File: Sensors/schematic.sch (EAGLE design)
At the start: 13 parts, among them IC1 LIS331DLHTR, IC2 BMI088, IC3 MCP9803T-M_MS, IC4 MS560702BA03-50

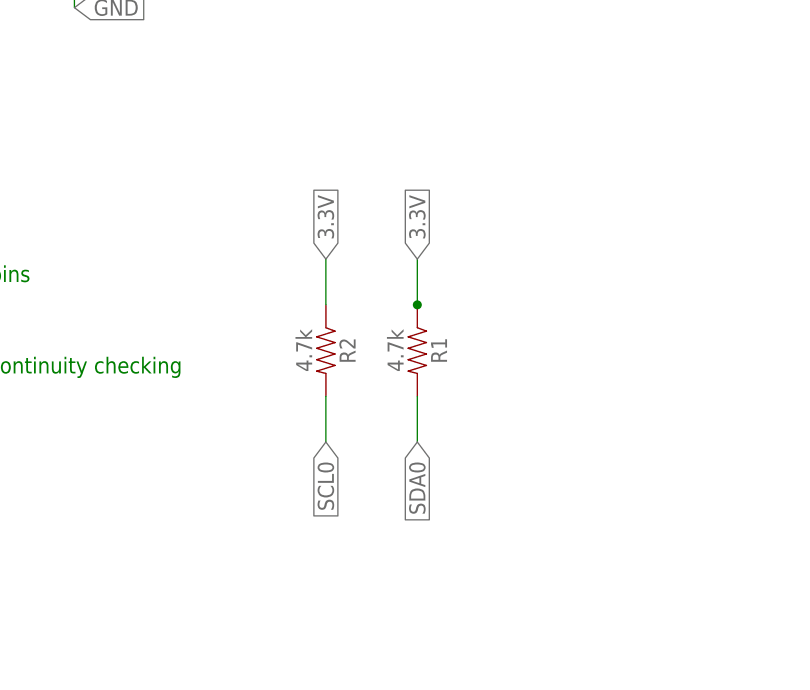
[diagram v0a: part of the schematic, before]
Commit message: Add files via upload
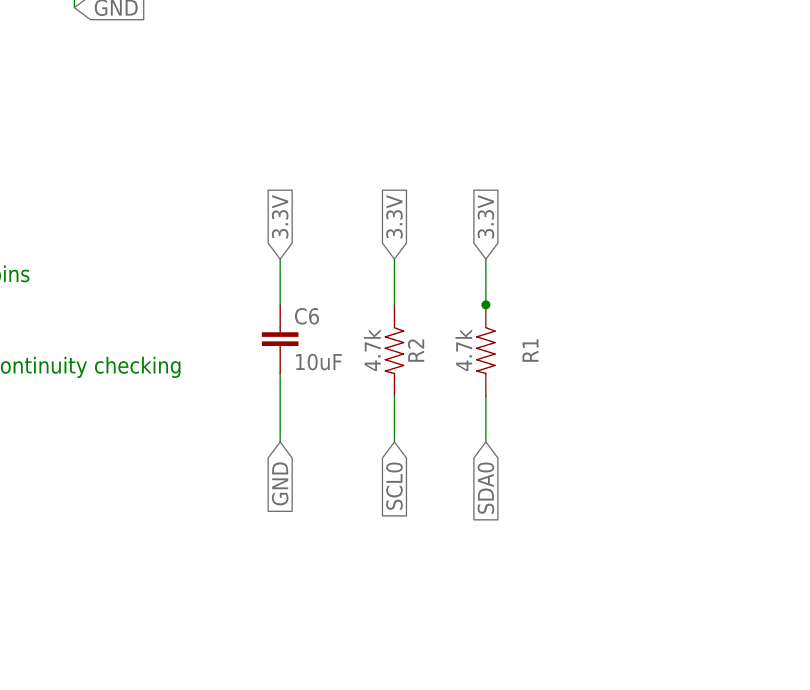
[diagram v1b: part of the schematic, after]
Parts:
- added C6: 10uF, SparkFun-Capacitors:10UF-0805-10V-10%
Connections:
- net 3.3V: now also C6.1
- net GND: now also C6.2
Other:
- moved on the sheet: R1, R2
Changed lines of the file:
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@@
 <part name="R2" library="SparkFun-Resistors" deviceset="RESISTOR" device="0805" value="4.7k"/>
 <part name="C4" library="875105240001" deviceset="875105240001" device=""/>
+<part name="C6" library="SparkFun-Capacitors" deviceset="10UF" device="-0805-10V-10%" value="10uF"/>
 </parts>
 <sheets>
@@
 <attribute name="DRAWING_NAME" x="165.1" y="19.05" size="2.54" layer="94"/>
 </instance>
-<instance part="R1" gate="G$1" x="132.08" y="38.1" smashed="yes" rot="R270">
-<attribute name="NAME" x="133.604" y="38.1" size="1.778" layer="95" font="vector" rot="R270" align="bottom-center"/>
-<attribute name="VALUE" x="130.556" y="38.1" size="1.778" layer="96" font="vector" rot="R270" align="top-center"/>
+<instance part="R1" gate="G$1" x="139.7" y="38.1" smashed="yes" rot="R270">
+<attribute name="NAME" x="143.764" y="38.1" size="1.778" layer="95" font="vector" rot="R270" align="bottom-center"/>
+<attribute name="VALUE" x="138.176" y="38.1" size="1.778" layer="96" font="vector" rot="R270" align="top-center"/>
 </instance>
 <instance part="C5" gate="G$1" x="93.98" y="93.98" smashed="yes" rot="R180">
@@
 <attribute name="VALUE" x="155.956" y="157.099" size="1.778" layer="96" font="vector" rot="R180"/>
 </instance>
-<instance part="R2" gate="G$1" x="121.92" y="38.1" smashed="yes" rot="R270">
-<attribute name="NAME" x="123.444" y="38.1" size="1.778" layer="95" font="vector" rot="R270" align="bottom-center"/>
-<attribute name="VALUE" x="120.396" y="38.1" size="1.778" layer="96" font="vector" rot="R270" align="top-center"/>
+<instance part="R2" gate="G$1" x="129.54" y="38.1" smashed="yes" rot="R270">
+<attribute name="NAME" x="131.064" y="38.1" size="1.778" layer="95" font="vector" rot="R270" align="bottom-center"/>
+<attribute name="VALUE" x="128.016" y="38.1" size="1.778" layer="96" font="vector" rot="R270" align="top-center"/>
 </instance>
 <instance part="C4" gate="G$1" x="218.44" y="88.9" smashed="yes" rot="R270">
 <attribute name="NAME" x="224.79" y="80.01" size="1.778" layer="95" rot="R270" align="center-left"/>
 <attribute name="VALUE" x="222.25" y="80.01" size="1.778" layer="96" rot="R270" align="center-left"/>
+</instance>
+<instance part="C6" gate="G$1" x="116.84" y="38.1" smashed="yes">
+<attribute name="NAME" x="118.364" y="41.021" size="1.778" layer="95" font="vector"/>
+<attribute name="VALUE" x="118.364" y="35.941" size="1.778" layer="96" font="vector"/>
 </instance>
 </instances>
@@
 <segment>
 <pinref part="R2" gate="G$1" pin="1"/>
-<wire x1="121.92" y1="43.18" x2="121.92" y2="48.26" width="0.1524" layer="91"/>
-<label x="121.92" y="48.26" size="1.778" layer="95" rot="R90" xref="yes"/>
+<wire x1="129.54" y1="43.18" x2="129.54" y2="48.26" width="0.1524" layer="91"/>
+<label x="129.54" y="48.26" size="1.778" layer="95" rot="R90" xref="yes"/>
 </segment>
 <segment>
 <pinref part="R1" gate="G$1" pin="1"/>
-<junction x="132.08" y="43.18"/>
-<wire x1="132.08" y1="43.18" x2="132.08" y2="48.26" width="0.1524" layer="91"/>
-<label x="132.08" y="48.26" size="1.778" layer="95" rot="R90" xref="yes"/>
+<junction x="139.7" y="43.18"/>
+<wire x1="139.7" y1="43.18" x2="139.7" y2="48.26" width="0.1524" layer="91"/>
+<label x="139.7" y="48.26" size="1.778" layer="95" rot="R90" xref="yes"/>
+</segment>
+<segment>
+<pinref part="C6" gate="G$1" pin="1"/>
+<wire x1="116.84" y1="43.18" x2="116.84" y2="48.26" width="0.1524" layer="91"/>
+<label x="116.84" y="48.26" size="1.778" layer="95" rot="R90" xref="yes"/>
 </segment>
 </net>
@@
 <label x="93.98" y="76.2" size="1.778" layer="95" xref="yes"/>
 </segment>
+<segment>
+<pinref part="C6" gate="G$1" pin="2"/>
+<wire x1="116.84" y1="35.56" x2="116.84" y2="27.94" width="0.1524" layer="91"/>
+<label x="116.84" y="27.94" size="1.778" layer="95" rot="R270" xref="yes"/>
+</segment>
 </net>
 <net name="SCL0" class="0">
@@
 <segment>
 <pinref part="R2" gate="G$1" pin="2"/>
-<wire x1="121.92" y1="33.02" x2="121.92" y2="27.94" width="0.1524" layer="91"/>
-<label x="121.92" y="27.94" size="1.778" layer="95" rot="R270" xref="yes"/>
+<wire x1="129.54" y1="33.02" x2="129.54" y2="27.94" width="0.1524" layer="91"/>
+<label x="129.54" y="27.94" size="1.778" layer="95" rot="R270" xref="yes"/>
 </segment>
 </net>
@@
 <segment>
 <pinref part="R1" gate="G$1" pin="2"/>
-<wire x1="132.08" y1="33.02" x2="132.08" y2="27.94" width="0.1524" layer="91"/>
-<label x="132.08" y="27.94" size="1.778" layer="95" rot="R270" xref="yes"/>
-</segment>
-</net>
+<wire x1="139.7" y1="33.02" x2="139.7" y2="27.94" width="0.1524" layer="91"/>
+<label x="139.7" y="27.94" size="1.778" layer="95" rot="R270" xref="yes"/>
+</segment>
+</net>
